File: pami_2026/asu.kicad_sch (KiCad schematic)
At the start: 20 parts, among them J2 Conn_01x03_Pin, J3 Conn_01x03_Pin, J4 Conn_01x03_Pin, J5 Conn_01x06, J6 Conn_01x06, J7 Conn_01x04_Pin, J8 Conn_01x04_Pin, SW1 SW_Reed

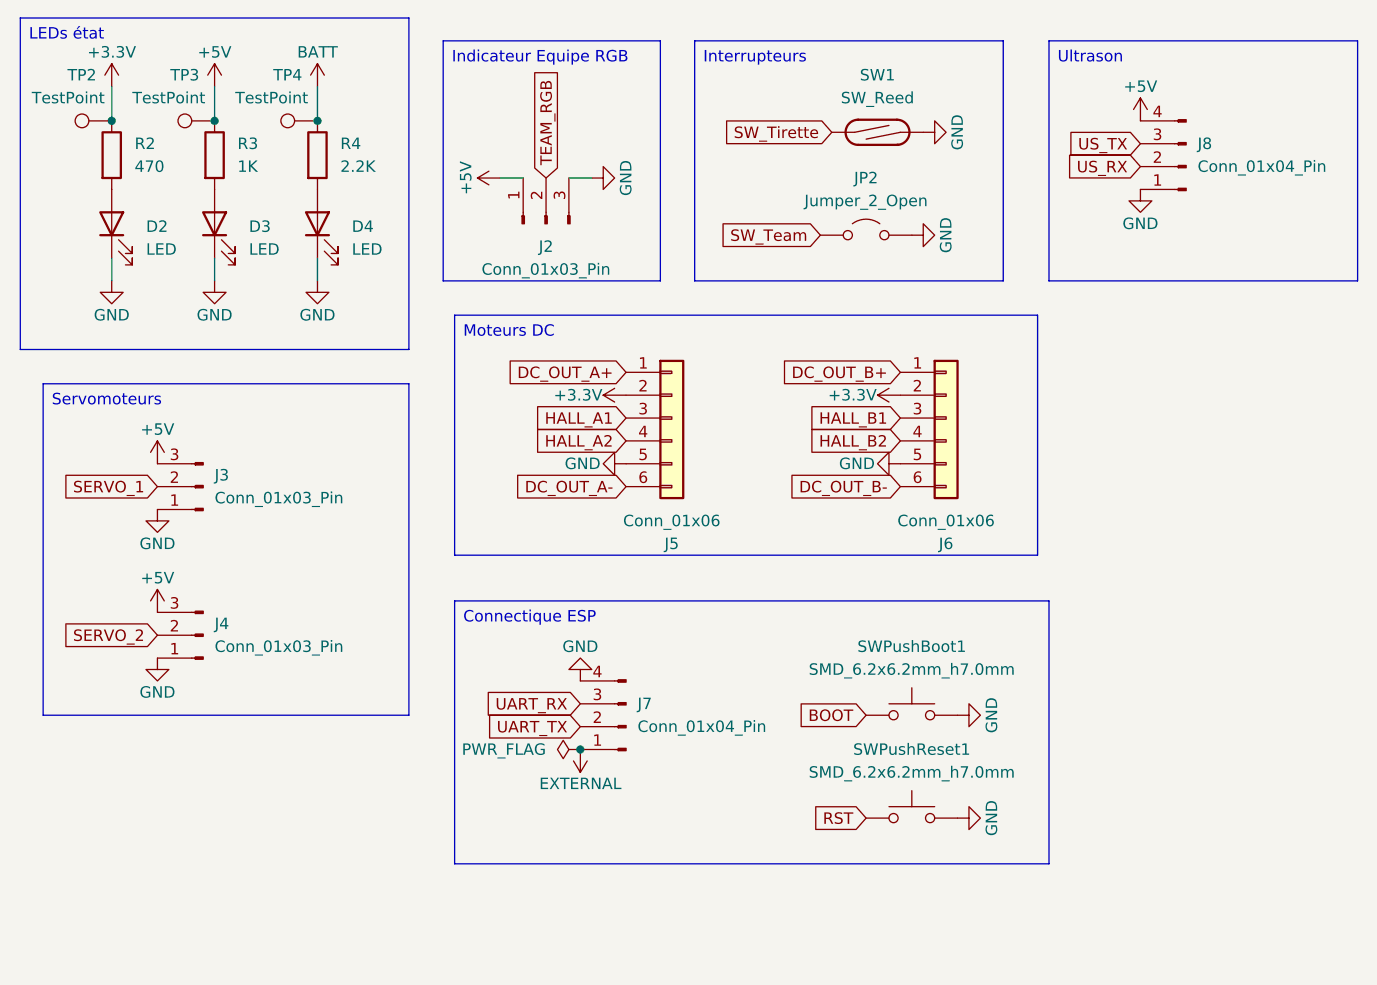
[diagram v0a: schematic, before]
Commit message: FEAT : Routing
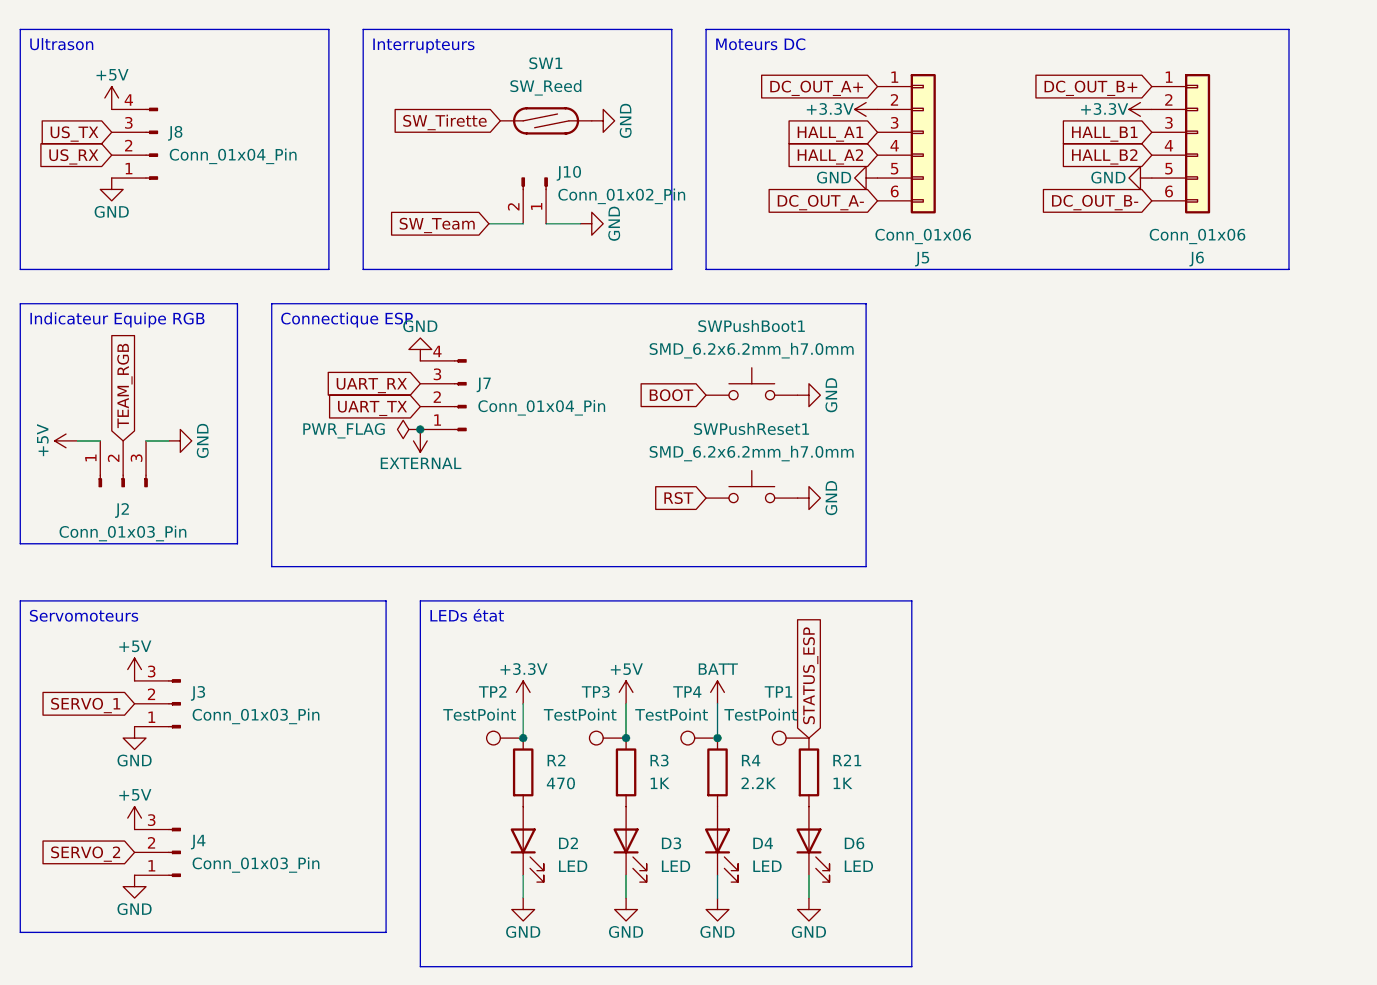
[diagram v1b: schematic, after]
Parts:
- removed JP2: Jumper_2_Open, Jumper:SolderJumper-2_P1.3mm_Open_RoundedPad1.0x1.5mm, symbol Jumper:Jumper_2_Open
- added D6: LED, LED_SMD:LED_0603_1608Metric, symbol Device:LED
- added J10: Conn_01x02_Pin, Connector_PinHeader_2.54mm:PinHeader_1x02_P2.54mm_Vertical, symbol Connector:Conn_01x02_Pin
- added R21: 1K, Resistor_SMD:R_0603_1608Metric, symbol Device:R
- added TP1: TestPoint, TestPoint:TestPoint_Pad_1.0x1.0mm, symbol Connector:TestPoint
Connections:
- net GND: now also D6.1 (K), J10.1 (Pin_1)
- net SW_Team: now also J10.2 (Pin_2)
- new net: D6.2 (A), R21.2
- new net STATUS_ESP: R21.1, TP1.1
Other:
- moved on the sheet: D2, D3, D4, J2, J3, J4, J5, J6, J7, J8, R2, R3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
